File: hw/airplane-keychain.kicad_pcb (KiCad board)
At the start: 2 copper layers, 100 x 75 mm, 18 parts, among them SW2 SPST, U1 ATtiny85-20P

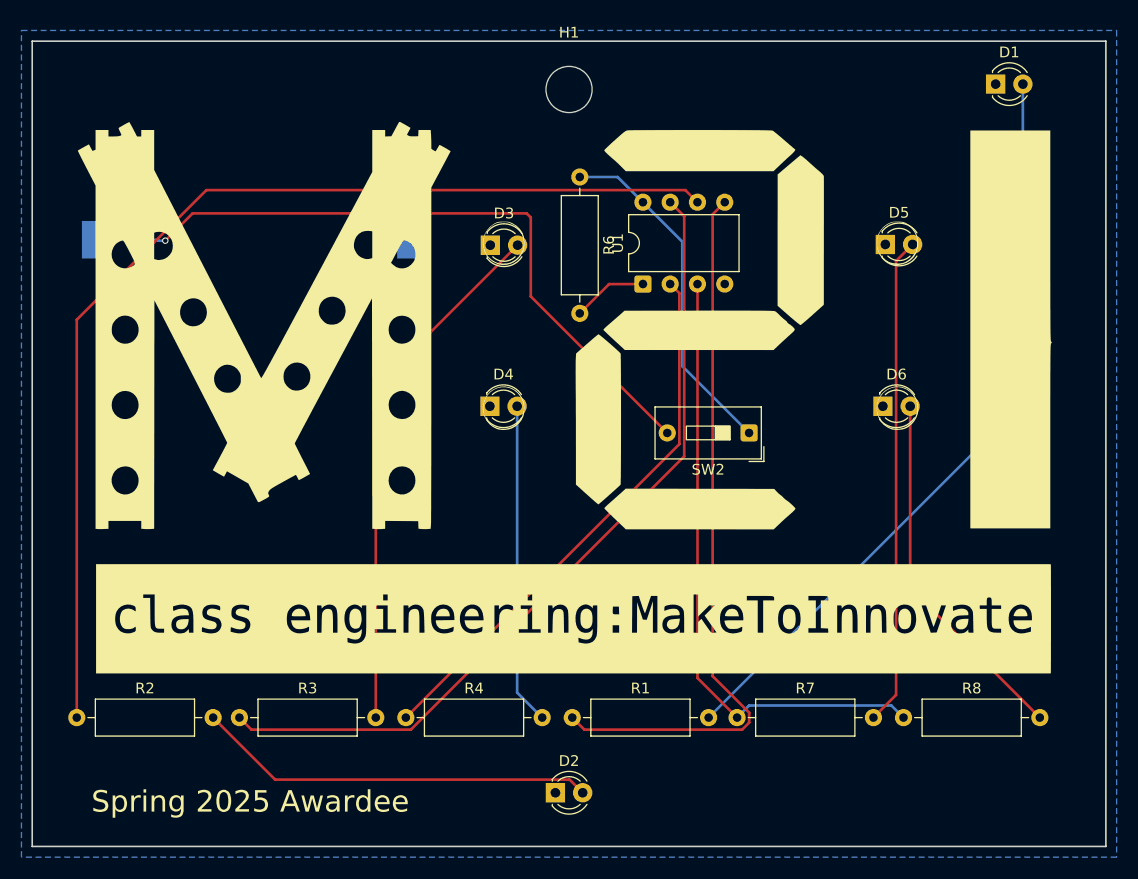
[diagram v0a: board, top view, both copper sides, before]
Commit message: Production Run
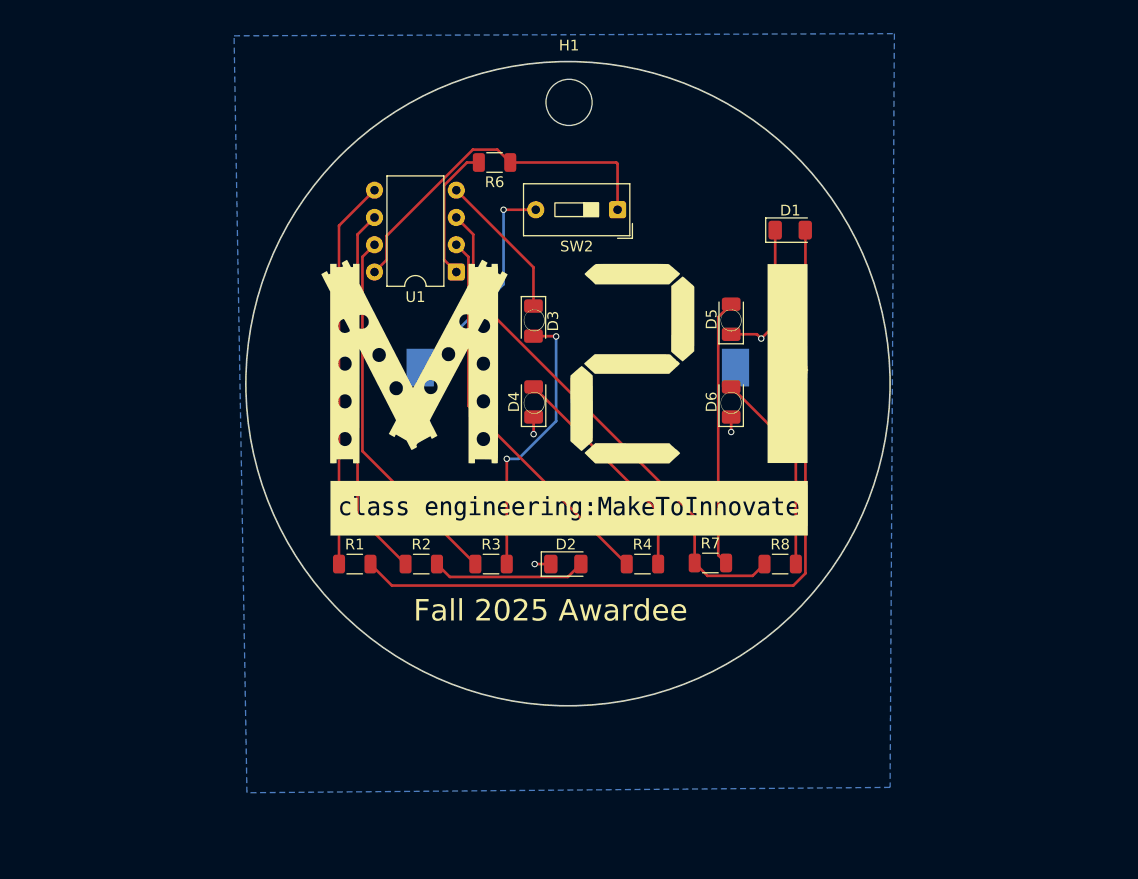
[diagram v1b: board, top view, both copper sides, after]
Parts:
- D1, D3, D4: value LED -> Red; footprint LED_THT:LED_D3.0mm -> LED_SMD:LED_1206_3216Metric
- D2, D5, D6: value LED -> Amber; footprint LED_THT:LED_D3.0mm -> LED_SMD:LED_1206_3216Metric
- R1, R2, R3, R4, R6, R7, R8: footprint Resistor_THT:R_Axial_DIN0309_L9.0mm_D3.2mm_P12.70mm_Horizontal -> Resistor_SMD:R_1206_3216Metric
- moved R2 35.1 mm to (136.2, 98.7)
- moved BT1 32.5 mm to (150.8, 80.4)
- moved R3 27.5 mm to (142.7, 98.7)
- moved R4 26.3 mm to (156.8, 98.7)
- moved R1 24.8 mm to (130.0, 98.7)
- moved SW2 24.1 mm to (154.5, 65.7)
- moved D1 23.5 mm to (170.6, 67.6)
- moved D2 21.3 mm to (149.7, 98.7)
- moved R8 18.3 mm to (169.7, 98.7)
- moved U1 17.4 mm to (139.5, 71.5), turned to 180 degrees
- moved D5 16.0 mm to (165.1, 75.9), turned to 90 degrees
- moved R7 14.6 mm to (163.2, 98.6)
- moved D6 14.1 mm to (165.1, 83.6), turned to 90 degrees
- moved D3 8.13 mm to (146.7, 76.1), turned to -90 degrees
- moved R6 8.05 mm to (143.1, 61.3), turned to 180 degrees
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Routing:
- net Net-(U1-PB1): track 100.3 -> 34.8 mm
- net Net-(BT1-+): track 67.1 -> 20.9 mm
- net Net-(U1-PB2): track 76.6 -> 34.6 mm
- net GND: track 0.33 -> 31.9 mm, vias 0 -> 4
- net Net-(U1-AREF/PB0): track 67.6 -> 36.2 mm
- net Net-(D3-A): track 49.5 -> 25.9 mm, vias 0 -> 2
- net Net-(D2-A): track 37.3 -> 14.4 mm
- net Net-(D5-A): track 45.6 -> 24.9 mm
- net Net-(D6-A): track 34.0 -> 19.0 mm
- net Net-(U1-XTAL1/PB3): track 51.3 -> 36.3 mm
- net Net-(U1-XTAL2/PB4): track 58.3 -> 48.8 mm
- net Net-(D4-A): track 30.0 -> 21.3 mm
- net Net-(U1-~{RESET}/PB5): track 7.01 -> 12.7 mm
- net Net-(D1-A): track 71.1 -> 73.8 mm
- net Net-(U1-VCC): track 32.4 -> 33.5 mm
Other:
- board size 100 x 75 mm -> 60 x 60 mm
- board text added: "Fall 2025 Awardee"
- board text removed: "Spring 2025 Awardee"
